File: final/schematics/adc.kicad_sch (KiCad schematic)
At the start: 6 parts, among them U10 LTC6903CMS8-TRPBF, U9 ADS131M02IPWR

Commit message: fixing issues
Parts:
- R29, R30, R31, R32: footprint (none) -> Resistor_SMD:R_0603_1608Metric
- U9: footprint footprints:TSSOP20_PW_TEX -> ADS131M02IPWR:TSSOP20_PW_TEX
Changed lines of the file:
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@@
 			)
 		)
-		(property "Footprint" ""
+		(property "Footprint" "Resistor_SMD:R_0603_1608Metric"
 			(at 235.712 66.04 90)
 			(hide yes)
@@
 			)
 		)
-		(property "Footprint" ""
+		(property "Footprint" "Resistor_SMD:R_0603_1608Metric"
 			(at 228.092 66.04 90)
 			(hide yes)
@@
 			)
 		)
-		(property "Footprint" "footprints:TSSOP20_PW_TEX"
+		(property "Footprint" "ADS131M02IPWR:TSSOP20_PW_TEX"
 			(at 148.59 53.34 0)
 			(hide yes)
@@
 			)
 		)
-		(property "Footprint" ""
+		(property "Footprint" "Resistor_SMD:R_0603_1608Metric"
 			(at 37.592 57.15 90)
 			(hide yes)
@@
 			)
 		)
-		(property "Footprint" ""
+		(property "Footprint" "Resistor_SMD:R_0603_1608Metric"
 			(at 221.742 66.04 90)
 			(hide yes)

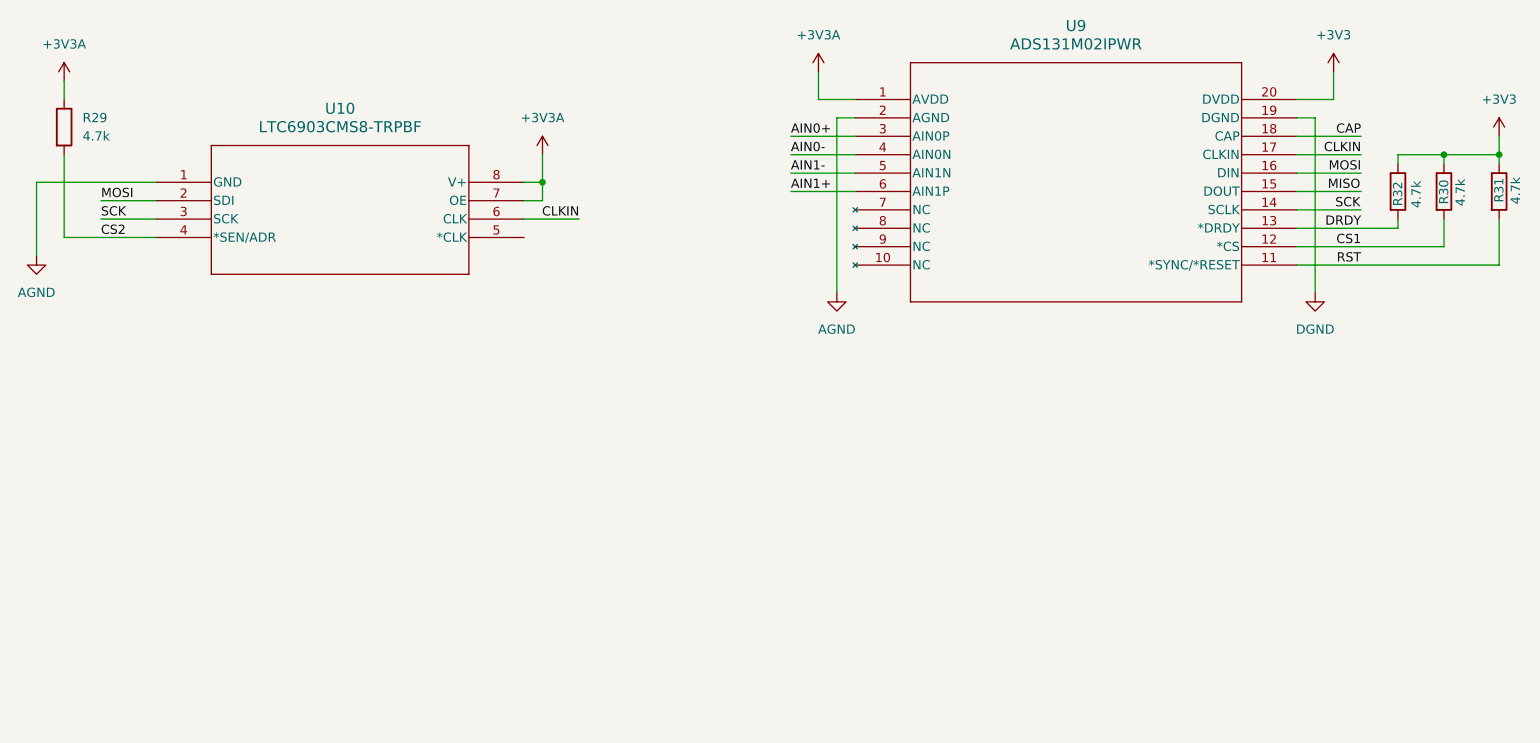
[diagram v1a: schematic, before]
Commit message: finishing
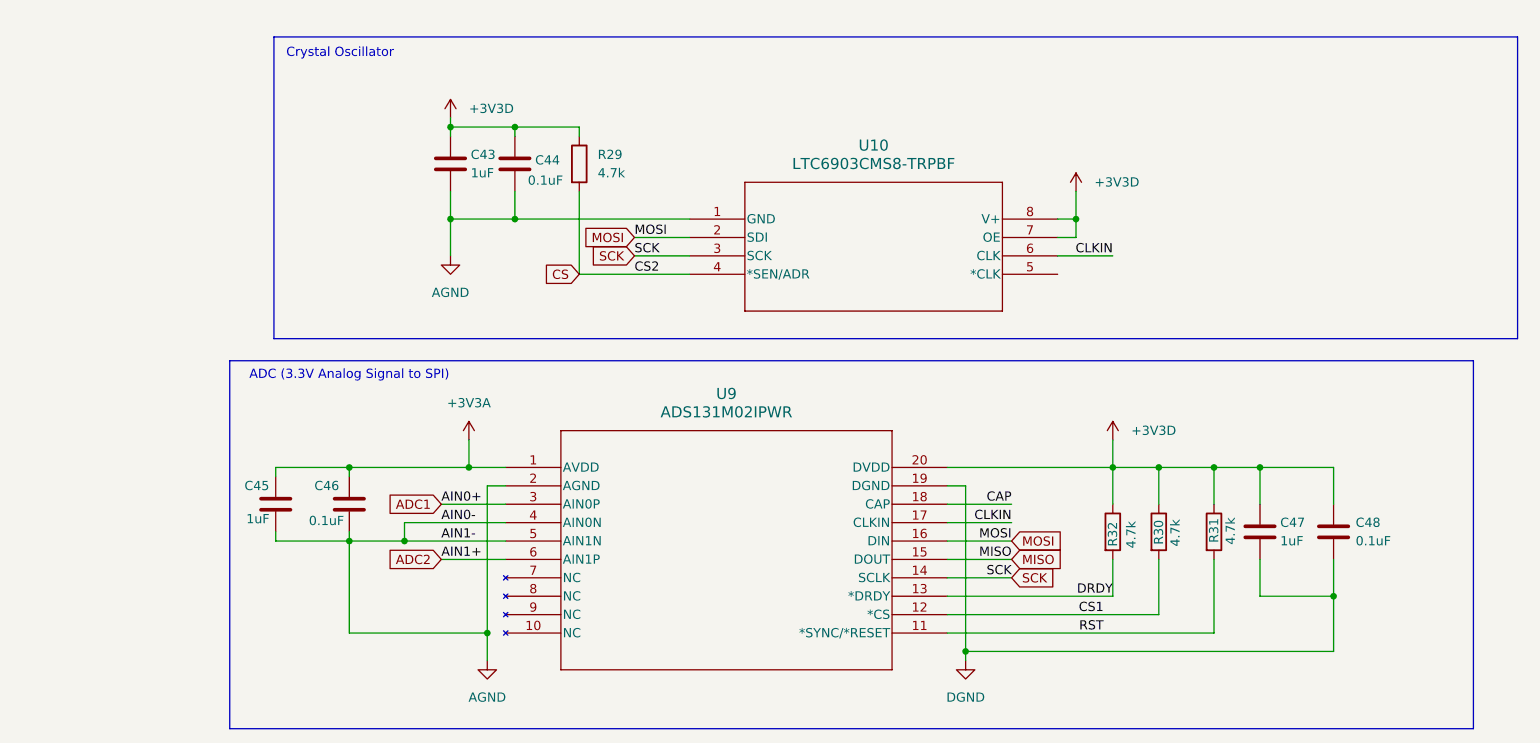
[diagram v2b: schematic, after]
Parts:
- added C43, C45, C47: 1uF, Capacitor_SMD:C_0603_1608Metric, symbol Device:C
- added C44, C46, C48: 0.1uF, Capacitor_SMD:C_0603_1608Metric, symbol Device:C
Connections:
- net AIN0- is gone; now on net AGND: U9.4 (AIN0N)
- net AIN1- is gone; now on net AGND: U9.5 (AIN1N)
- net +3V3A: now also C45.1, C46.1; no longer R29.1, U10.7 (OE), U10.8 (V+)
- net AGND: now also C43.2, C44.2, C45.2, C46.2
- net DGND: now also C47.2, C48.2
- net +3V3 renamed +3V3D
- net +3V3D: now also R29.1, U10.7 (OE), U10.8 (V+), C43.1, C44.1, C47.1, C48.1
- net AIN0+ renamed ADC1
- net AIN1+ renamed ADC2
- net CS2 renamed CS
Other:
- note added: "ADC (3.3V Analog Signal to SPI)"
- note added: "Crystal Oscillator"
- moved on the sheet: R29, R30, R31, R32, U10, U9
